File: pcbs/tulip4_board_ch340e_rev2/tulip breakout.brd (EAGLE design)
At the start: 81.1 x 46 mm, 59 parts, among them IC1 MCP73831/OT, J1 CSP-USC16-TR, U1 ESP32-S3-WROOM-2-N32R8V, U2 LD29150DT33R, U3 PCM5101APW, U6 CH340C, X2 FH12-40S-0.5SH

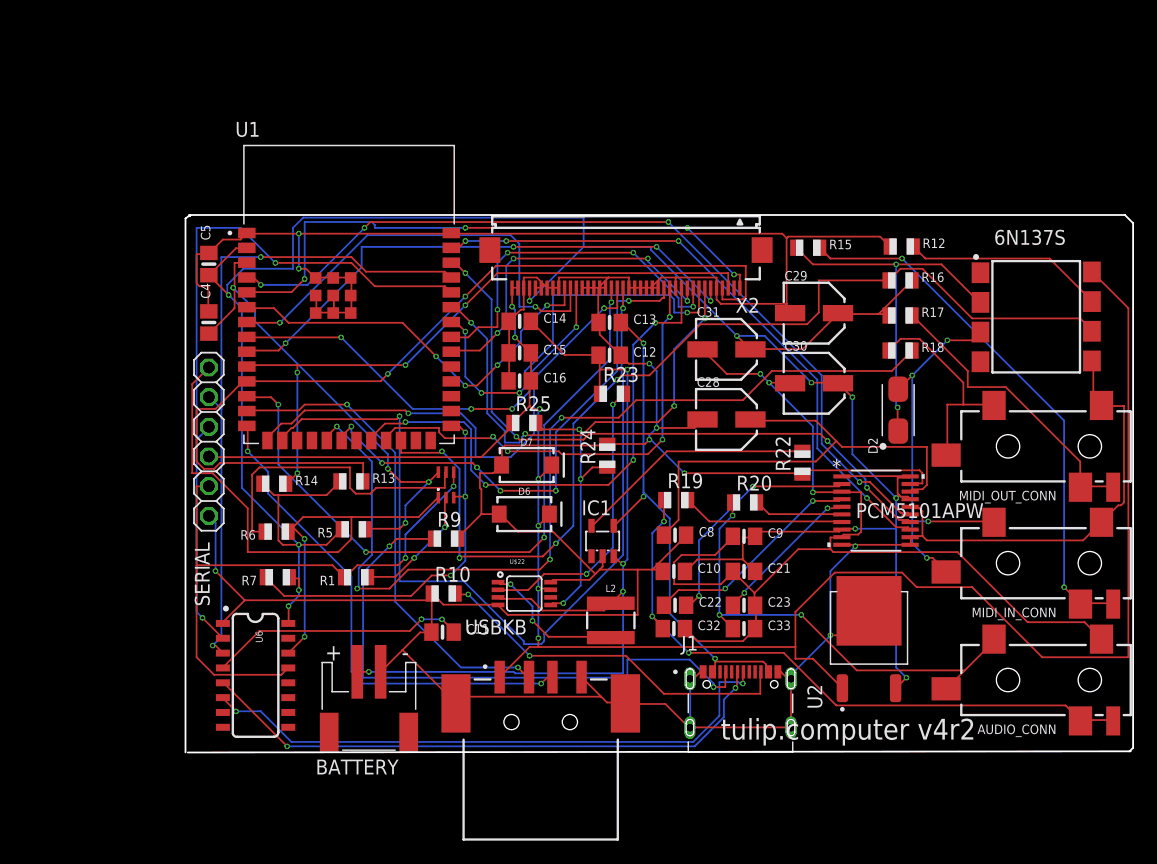
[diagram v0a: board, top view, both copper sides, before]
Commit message: .
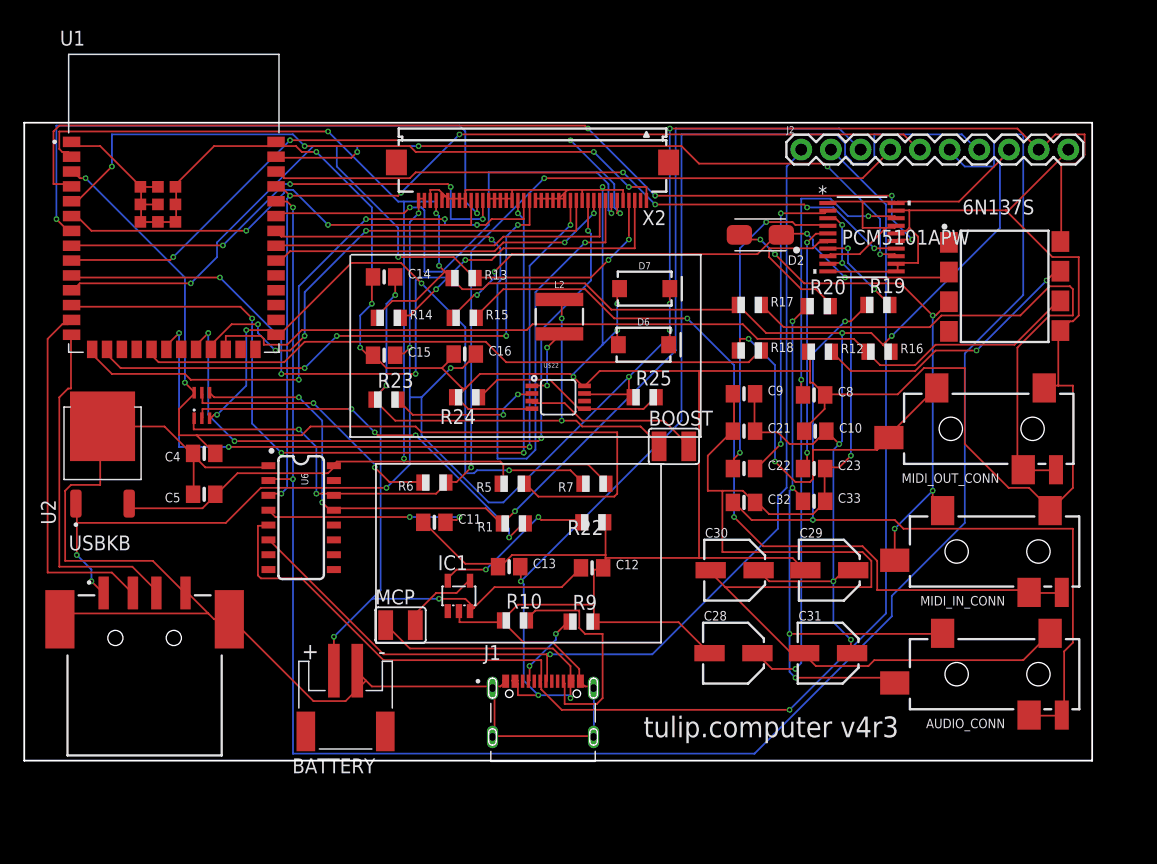
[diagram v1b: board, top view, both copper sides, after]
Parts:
- removed SERIAL: (no value), adafruit:1X06
- added BOOST, MCP: (no value), jumper:SJW
- added J2: (no value), SparkFun-Connectors:1X10
- moved U2 67.5 mm to (6.70, 26.1)
- moved USBKB 34.7 mm to (10.3, 10.4)
- moved R15 30.0 mm to (37.7, 37.8)
- moved R7 28.3 mm to (48.8, 23.6)
- moved C31 27.4 mm to (68.8, 9.10)
- moved L2 26.4 mm to (45.8, 37.9)
- moved R19 24.0 mm to (73.1, 38.9)
- moved U3 23.4 mm to (71.7, 44.7)
- moved C13 22.6 mm to (41.5, 16.5)
- moved C29 22.0 mm to (68.9, 16.2)
- moved RESET 22.0 mm to (15.2, 30.3)
- moved C28 20.0 mm to (60.7, 9.10)
- moved R13 19.9 mm to (37.6, 41.2)
- moved C5 19.7 mm to (15.4, 22.7), turned to 180 degrees
- moved R23 19.3 mm to (31.0, 30.8)
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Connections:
- new net N$4: IC1.4, MCP.2
- new net N$5: BOOST.2, U$22.3
- net !DTR: now also J2.3; no longer SERIAL.2
- net !RTS: now also J2.4; no longer SERIAL.6
- net 3V3: now also J2.8
- net 5V: now also J2.9; no longer SERIAL.3
- net 5V_USB: now also J2.7, MCP.1; no longer IC1.4
- net DN1: now also J2.1
- net DP1: now also J2.2
- net GND: now also J2.10; no longer SERIAL.1
- net UART0_RXD: now also J2.6; no longer SERIAL.4
- net UART0_TXD: now also J2.5; no longer SERIAL.5
- net VBATT: now also BOOST.1; no longer U$22.3
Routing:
- net UART0_RXD: track 61.7 -> 161.9 mm
- net 5V_USB: track 43.1 -> 112.7 mm
- net GND: track 402.9 -> 467.4 mm, vias 9 -> 7
- net DP1: track 50.7 -> 110.3 mm, vias 2 -> 1
- net 3V3: track 209.8 -> 261.0 mm, vias 11 -> 9
- net N$42: track 51.2 -> 6.66 mm
- net ESP32_EN: track 42.3 -> 81.8 mm, vias 4 -> 2
- net !DTR: track 52.4 -> 90.5 mm, vias 2 -> 3
- net DN1: track 51.0 -> 87.7 mm, vias 2 -> 1
- net !RTS: track 57.0 -> 88.4 mm, vias 2 -> 4
- net VSYNC: track 36.1 -> 66.4 mm, vias 4 -> 2
- net UART0_TXD: track 56.6 -> 85.1 mm, vias 2 -> 4
- net MIDI_OUT_SOURCE: track 25.4 -> 51.0 mm
- net MIDI_IN_SOURCE: track 46.2 -> 71.2 mm
- net MIDI_OUT: track 79.7 -> 54.8 mm, vias 4 -> 0
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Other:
- board size 81.1 x 46 mm -> 91.4 x 54.6 mm
- board text added: "tulip.computer v4r3"
- board text removed: "tulip.computer v4r2"
